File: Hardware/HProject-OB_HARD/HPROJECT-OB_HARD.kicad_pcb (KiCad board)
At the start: 2 copper layers, 54.8 x 34.5 mm, 18 parts, among them J1 PWR, J2 Hrn_Ctrl, J3 Hrn_Out1, J4 Hrn_Out2, M1 MPMOS

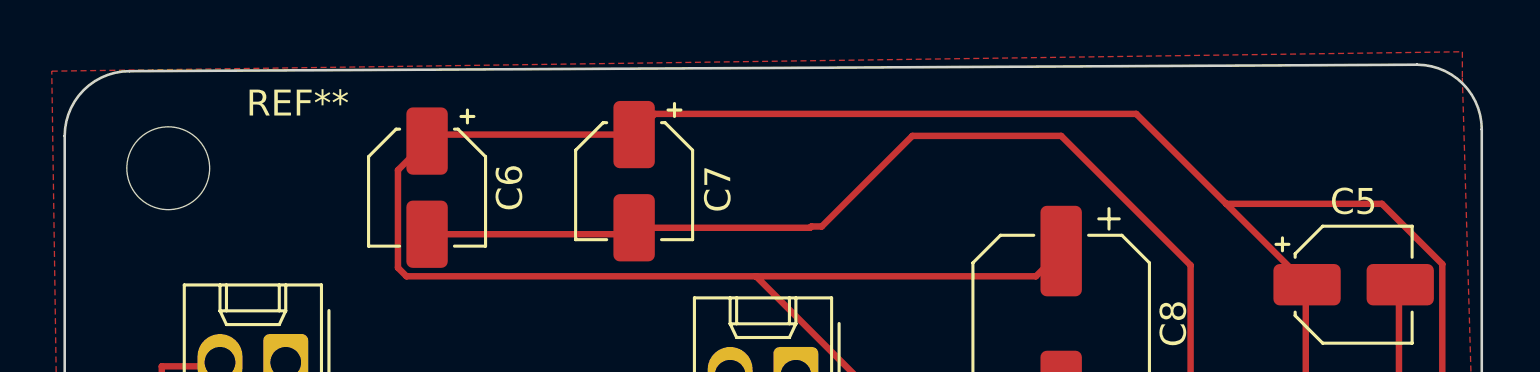
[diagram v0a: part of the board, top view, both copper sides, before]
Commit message: onboarding project fixes
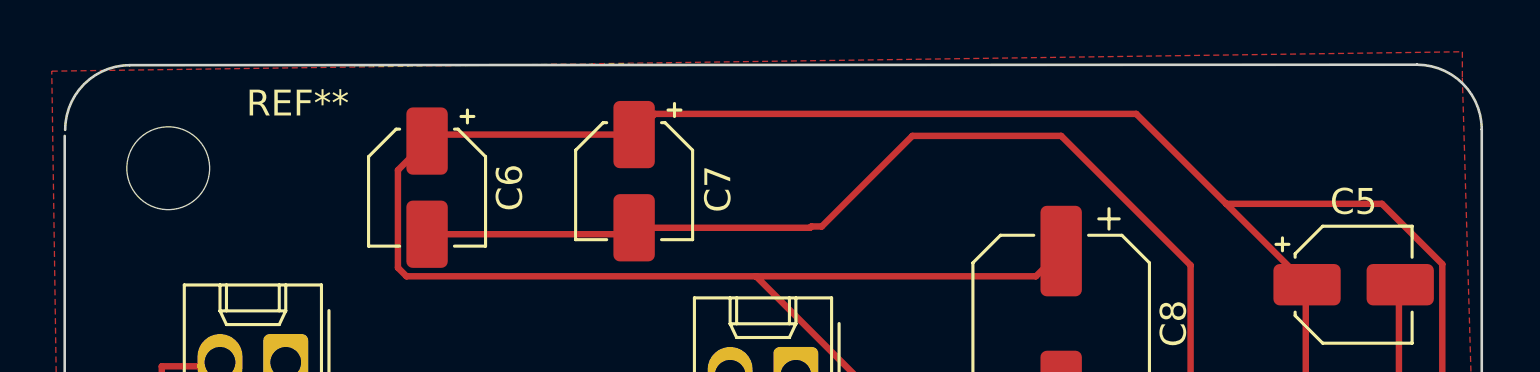
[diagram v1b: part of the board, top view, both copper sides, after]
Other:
- outline, holes or cut-outs redrawn
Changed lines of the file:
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@@
 	)
 	(gr_arc
-		(start 139.5 87.75)
-		(mid 140.232233 85.982233)
-		(end 142 85.25)
+		(start 139.517767 87.517767)
+		(mid 140.25 85.75)
+		(end 142.017767 85.017767)
 		(stroke
 			(width 0.1)
@@
 	)
 	(gr_line
-		(start 191.75 85)
-		(end 142 85.25)
+		(start 142.0178 85.017767)
+		(end 191.75 85)
 		(stroke
 			(width 0.1)
@@
 		(layer "Edge.Cuts")
 	)
+	(dimension
+		(type orthogonal)
+		(layer "F.Fab")
+		(pts
+			(xy 177.75 85) (xy 177.75 119.5)
+		)
+		(height 33.25)
+		(orientation 1)
+		(format
+			(prefix "")
+			(suffix "")
+			(units 3)
+			(units_format 1)
+			(precision 4)
+		)
+		(style
+			(thickness 0.1)
+			(arrow_length 1.27)
+			(text_position_mode 0)
+			(arrow_direction outward)
+			(extension_height 0.58642)
+			(extension_offset 0.5)
+			(keep_text_aligned yes)
+		)
+		(gr_text "34.5000 mm"
+			(at 209.85 102.25 90)
+			(layer "F.Fab")
+			(effects
+				(font
+					(size 1 1)
+					(thickness 0.15)
+				)
+			)
+		)
+	)
+	(dimension
+		(type orthogonal)
+		(layer "F.Fab")
+		(pts
+			(xy 188 114.5) (xy 143.5 89)
+		)
+		(height -54.75)
+		(orientation 1)
+		(format
+			(prefix "")
+			(suffix "")
+			(units 3)
+			(units_format 1)
+			(precision 4)
+		)
+		(style
+			(thickness 0.1)
+			(arrow_length 1.27)
+			(text_position_mode 0)
+			(arrow_direction outward)
+			(extension_height 0.58642)
+			(extension_offset 0.5)
+			(keep_text_aligned yes)
+		)
+		(gr_text "25.5000 mm"
+			(at 132.1 101.75 90)
+			(layer "F.Fab")
+			(effects
+				(font
+					(size 1 1)
+					(thickness 0.15)
+				)
+			)
+		)
+	)
+	(dimension
+		(type orthogonal)
+		(layer "F.Fab")
+		(pts
+			(xy 194.25 94.55) (xy 139.5 94.5)
+		)
+		(height -15.3)
+		(orientation 0)
+		(format
+			(prefix "")
+			(suffix "")
+			(units 3)
+			(units_format 1)
+			(precision 4)
+		)
+		(style
+			(thickness 0.1)
+			(arrow_length 1.27)
+			(text_position_mode 0)
+			(arrow_direction outward)
+			(extension_height 0.58642)
+			(extension_offset 0.5)
+			(keep_text_aligned yes)
+		)
+		(gr_text "54.7500 mm"
+			(at 166.875 78.1 0)
+			(layer "F.Fab")
+			(effects
+				(font
+					(size 1 1)
+					(thickness 0.15)
+				)
+			)
+		)
+	)
+	(dimension
+		(type orthogonal)
+		(layer "F.Fab")
+		(pts
+			(xy 143.5 89) (xy 188 114.5)
+		)
+		(height 34)
+		(orientation 0)
+		(format
+			(prefix "")
+			(suffix "")
+			(units 3)
+			(units_format 1)
+			(precision 4)
+		)
+		(style
+			(thickness 0.1)
+			(arrow_length 1.27)
+			(text_position_mode 0)
+			(arrow_direction outward)
+			(extension_height 0.58642)
+			(extension_offset 0.5)
+			(keep_text_aligned yes)
+		)
+		(gr_text "44.5000 mm"
+			(at 165.75 121.85 0)
+			(layer "F.Fab")
+			(effects
+				(font
+					(size 1 1)
+					(thickness 0.15)
+				)
+			)
+		)
+	)
 	(segment

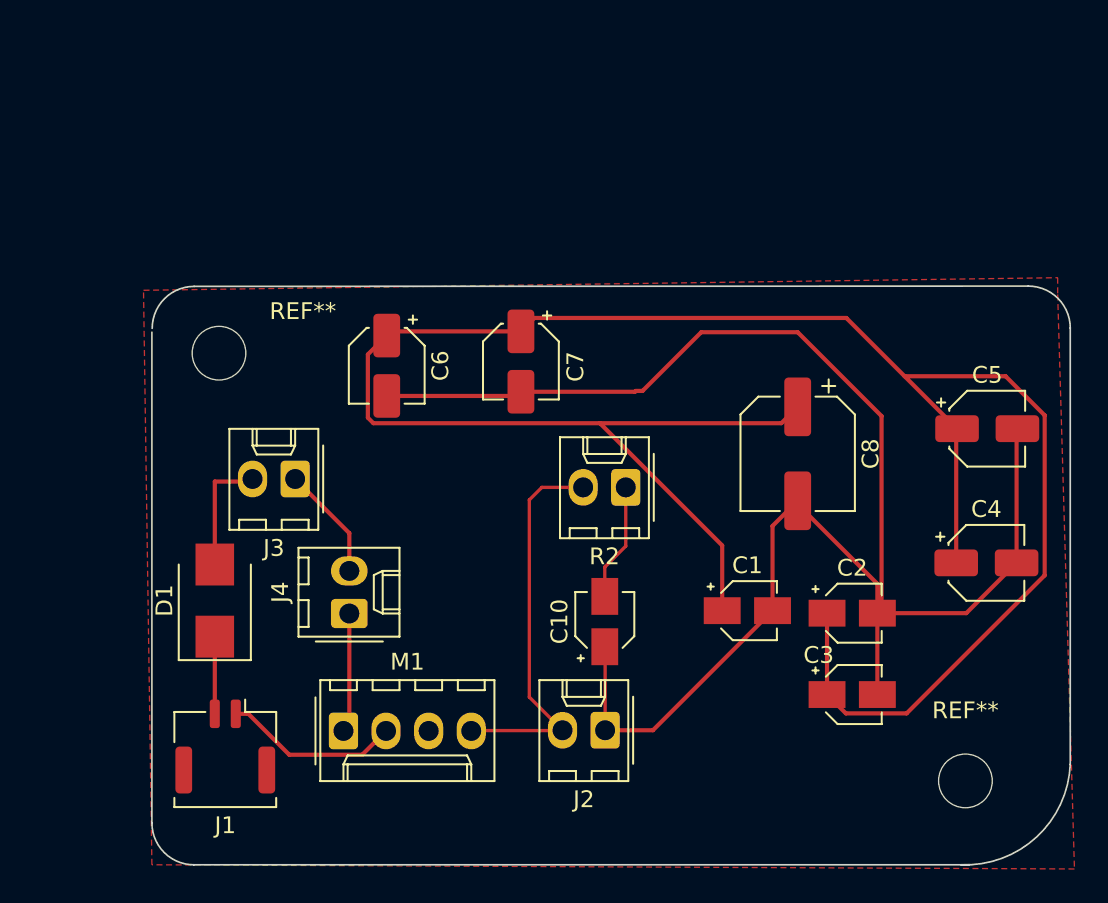
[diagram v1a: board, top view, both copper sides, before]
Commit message: Glingle Onboarding Projects - updated
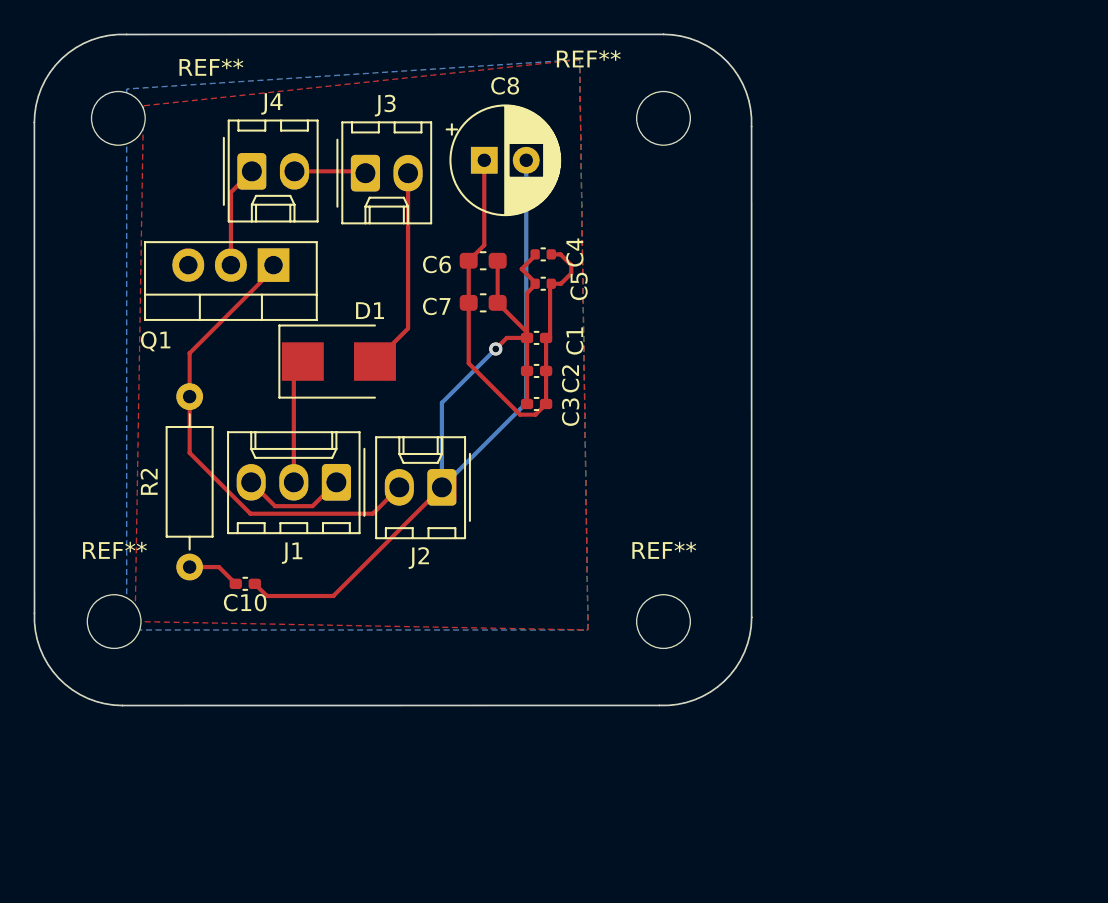
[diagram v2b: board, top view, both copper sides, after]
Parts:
- removed M1: MPMOS, Connector_Molex:Molex_KK-254_AE-6410-04A_1x04_P2.54mm_Vertical
- removed the REF** at (188.0, 114.5)
- removed the REF** at (143.5, 89.0)
- added Q1: IRF740, Package_TO_SOT_THT:TO-220-3_Vertical, F.Cu at (146.8, 83.8)
- added REF**: MountingHole_3.2mm_M3, MountingHole:MountingHole_3.2mm_M3, F.Cu at (137.2, 105.0)
- added REF**: MountingHole_3.2mm_M3, MountingHole:MountingHole_3.2mm_M3, F.Cu at (170.0, 75.0)
- added REF**: MountingHole_3.2mm_M3, MountingHole:MountingHole_3.2mm_M3, F.Cu at (170.0, 105.0)
- added REF**: MountingHole_3.2mm_M3, MountingHole:MountingHole_3.2mm_M3, F.Cu at (137.5, 75.0)
- C1, C10, C2, C3: footprint Capacitor_SMD:CP_Elec_3x5.3 -> Capacitor_SMD:C_0402_1005Metric_Pad0.74x0.62mm_HandSolder
- C4, C5: footprint Capacitor_SMD:CP_Elec_4x3 -> Capacitor_SMD:C_0402_1005Metric
- C6, C7: footprint Capacitor_SMD:CP_Elec_4x5.3 -> Capacitor_SMD:C_0603_1608Metric_Pad1.08x0.95mm_HandSolder
- C8: footprint Capacitor_SMD:CP_Elec_6.3x5.4 -> Capacitor_THT:CP_Radial_D6.3mm_P2.50mm
- J1: footprint Connector_Molex:Molex_CLIK-Mate_502382-0270_1x02-1MP_P1.25mm_Vertical -> Connector_Molex:Molex_KK-254_AE-6410-03A_1x03_P2.54mm_Vertical
- R2: value R -> 1K ohm; footprint Connector_Molex:Molex_KK-254_AE-6410-02A_1x02_P2.54mm_Vertical -> Resistor_THT:R_Axial_DIN0207_L6.3mm_D2.5mm_P10.16mm_Horizontal
- moved C4 32.2 mm to (162.8, 83.1), turned to 180 degrees
- moved C5 27.8 mm to (162.8, 84.9), turned to 180 degrees
- moved J4 27.0 mm to (145.5, 78.2), turned to 0 degrees
- moved R2 26.4 mm to (141.8, 101.8), turned to 90 degrees
- moved C8 25.6 mm to (159.3, 77.5), turned to 0 degrees
- moved C3 25.6 mm to (162.4, 92.0), turned to 180 degrees
- moved C2 23.7 mm to (162.4, 90.1), turned to 180 degrees
- moved C10 21.6 mm to (145.1, 102.8), turned to 180 degrees
- moved C1 20.6 mm to (162.4, 88.1), turned to 180 degrees
- moved J3 18.7 mm to (152.2, 78.3), turned to 0 degrees
- moved J2 17.4 mm to (156.8, 97.0)
- moved J1 17.1 mm to (150.5, 96.7)
- moved D1 16.1 mm to (150.7, 89.5), turned to 0 degrees
- moved C6 8.50 mm to (159.2, 83.5), turned to 180 degrees
- moved C7 4.16 mm to (159.2, 86.0), turned to 0 degrees
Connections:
- C6 pad 1: +24V -> GND
- C6 pad 2: GND -> +24V
- J1 pad 1: Net-(J1-Pin_1) -> GND
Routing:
- net +24V: track 131.5 -> 29.4 mm
- net /HornSignal: track 0.00 -> 27.9 mm
- net GND: track 96.2 -> 68.9 mm, vias 0 -> 1
- net Net-(J1-Pin_1): track 10.6 -> 0.00 mm
- net Net-(D1-A): track 7.26 -> 12.0 mm
- net Net-(C10-Pad2): track 0.00 -> 3.16 mm
- net Net-(D1-K): track 4.60 -> 7.42 mm
- net Net-(J3-Pin_1): track 6.82 -> 4.28 mm
- net /Horn In: track 7.14 -> 6.11 mm
- added copper zone on B.Cu, net GND
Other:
- board size 54.8 x 34.5 mm -> 42.8 x 40 mm
